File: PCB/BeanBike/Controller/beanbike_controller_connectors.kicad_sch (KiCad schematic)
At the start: 12 parts, among them J2 Motor Conn, J3 Throttle Conn, J4 PAS Conn, J5 Display Conn, J6 Brake Conn, J7 DEBUG Conn

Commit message: Footprints
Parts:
- J2: footprint (none) -> Connector_PinHeader_2.54mm:PinHeader_1x08_P2.54mm_Vertical
- J3, J4, J7: footprint (none) -> Connector_PinHeader_2.54mm:PinHeader_1x03_P2.54mm_Vertical
- J5: footprint (none) -> Connector_PinHeader_2.54mm:PinHeader_1x06_P2.54mm_Vertical
- J6: footprint (none) -> Connector_PinHeader_2.54mm:PinHeader_1x02_P2.54mm_Vertical
- R10, R6, R8: footprint (none) -> Resistor_SMD:R_0805_2012Metric; LCSC C98220 -> C17414
- R11, R7, R9: footprint (none) -> Resistor_SMD:R_0805_2012Metric; LCSC C137655 -> C17506
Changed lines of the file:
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@@
 			)
 		)
-		(property "Footprint" ""
+		(property "Footprint" "Resistor_SMD:R_0805_2012Metric"
 			(at 212.598 27.94 90)
 			(effects
@@
 			)
 		)
-		(property "LCSC" "C137655"
+		(property "LCSC" "C17506"
 			(at 210.82 27.94 0)
 			(effects
@@
 			)
 		)
-		(property "Footprint" ""
+		(property "Footprint" "Resistor_SMD:R_0805_2012Metric"
 			(at 211.328 48.26 90)
 			(effects
@@
 			)
 		)
-		(property "LCSC" "C137655"
+		(property "LCSC" "C17506"
 			(at 209.55 48.26 0)
 			(effects
@@
 			)
 		)
-		(property "Footprint" ""
+		(property "Footprint" "Resistor_SMD:R_0805_2012Metric"
 			(at 199.39 53.848 90)
 			(effects
@@
 			)
 		)
-		(property "LCSC" "C98220"
+		(property "LCSC" "C17414"
 			(at 199.39 52.07 90)
 			(effects
@@
 			)
 		)
-		(property "Footprint" ""
+		(property "Footprint" "Resistor_SMD:R_0805_2012Metric"
 			(at 200.66 33.528 90)
 			(effects
@@
 			)
 		)
-		(property "LCSC" "C98220"
+		(property "LCSC" "C17414"
 			(at 200.66 31.75 90)
 			(effects
@@
 			)
 		)
-		(property "Footprint" ""
+		(property "Footprint" "Connector_PinHeader_2.54mm:PinHeader_1x08_P2.54mm_Vertical"
 			(at 54.61 139.7 0)
 			(effects
@@
 			)
 		)
-		(property "Footprint" ""
+		(property "Footprint" "Connector_PinHeader_2.54mm:PinHeader_1x03_P2.54mm_Vertical"
 			(at 121.92 139.7 0)
 			(effects
@@
 			)
 		)
-		(property "Footprint" ""
+		(property "Footprint" "Connector_PinHeader_2.54mm:PinHeader_1x03_P2.54mm_Vertical"
 			(at 92.71 139.7 0)
 			(effects
@@
 			)
 		)
-		(property "Footprint" ""
+		(property "Footprint" "Connector_PinHeader_2.54mm:PinHeader_1x02_P2.54mm_Vertical"
 			(at 186.69 139.7 0)
 			(effects
@@
 			)
 		)
-		(property "Footprint" ""
+		(property "Footprint" "Resistor_SMD:R_0805_2012Metric"
 			(at 199.39 71.628 90)
 			(effects
@@
 			)
 		)
-		(property "LCSC" "C98220"
+		(property "LCSC" "C17414"
 			(at 199.39 69.85 90)
 			(effects
@@
 			)
 		)
-		(property "Footprint" ""
+		(property "Footprint" "Resistor_SMD:R_0805_2012Metric"
 			(at 211.328 66.04 90)
 			(effects
@@
 			)
 		)
-		(property "LCSC" "C137655"
+		(property "LCSC" "C17506"
 			(at 209.55 66.04 0)
 			(effects
@@
 			)
 		)
-		(property "Footprint" ""
+		(property "Footprint" "Connector_PinHeader_2.54mm:PinHeader_1x06_P2.54mm_Vertical"
 			(at 156.21 139.7 0)
 			(effects
@@
 			)
 		)
-		(property "Footprint" ""
+		(property "Footprint" "Connector_PinHeader_2.54mm:PinHeader_1x03_P2.54mm_Vertical"
 			(at 217.17 139.7 0)
 			(effects

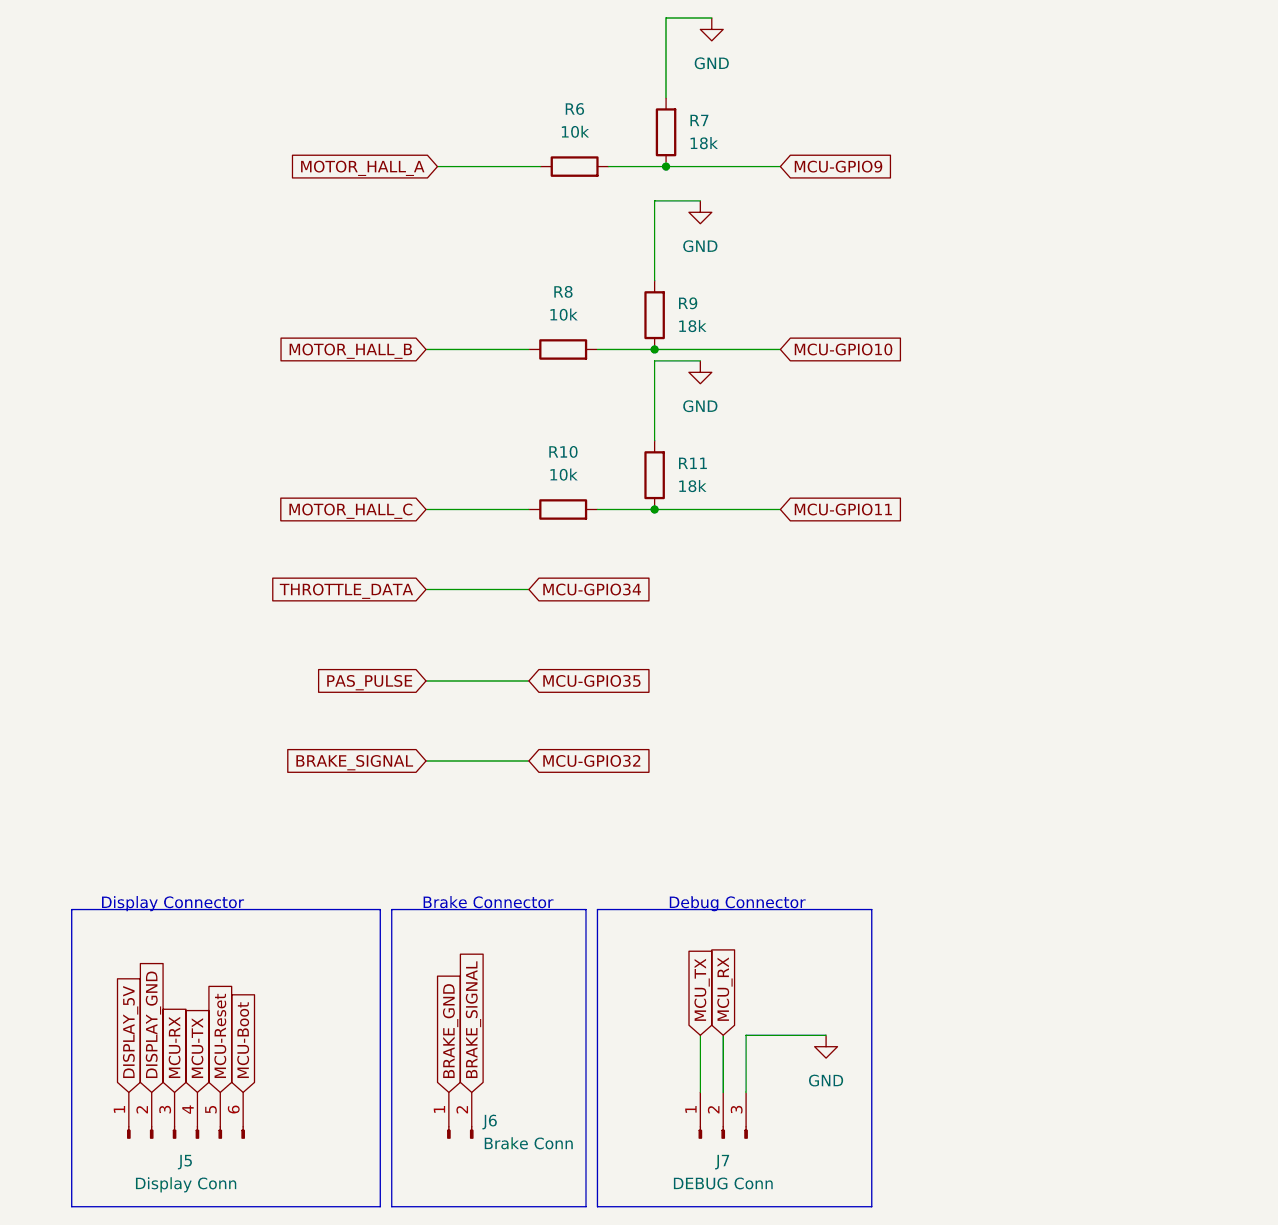
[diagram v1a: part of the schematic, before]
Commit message: PCB v3
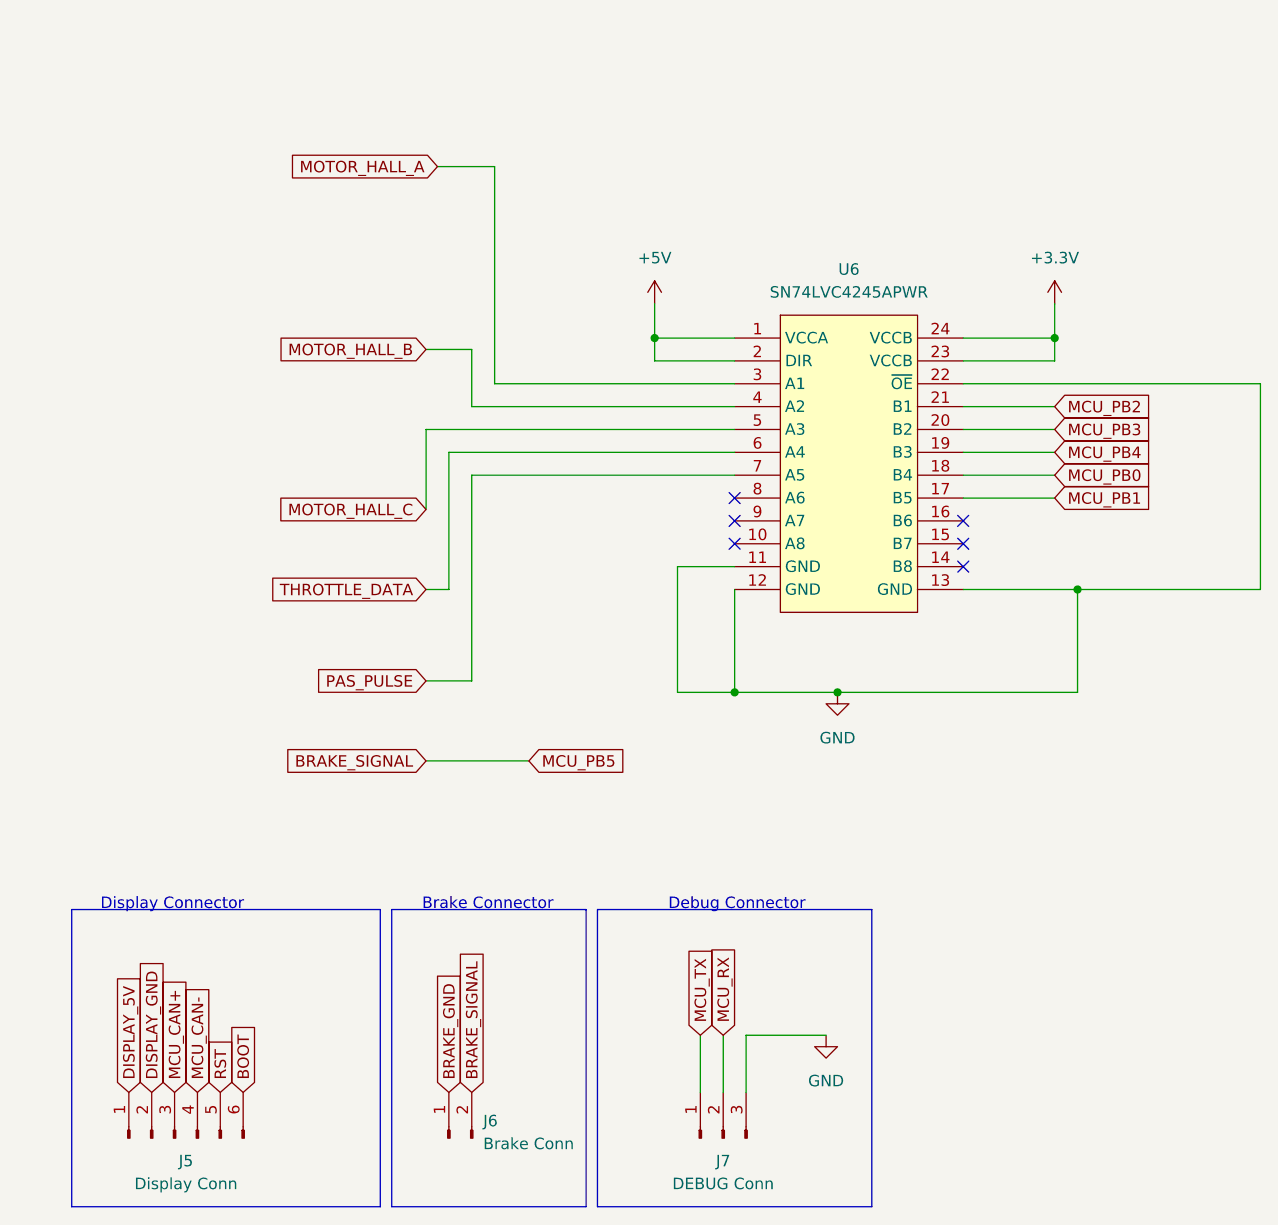
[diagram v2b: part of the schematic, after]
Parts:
- removed R10, R6, R8: 10k, Resistor_SMD:R_0805_2012Metric, symbol Device:R
- removed R11, R7, R9: 18k, Resistor_SMD:R_0805_2012Metric, symbol Device:R
- added U6: SN74LVC4245APWR, easyeda2kicad:TSSOP-24_L7.8-W4.4-P0.65-LS6.4-BL, symbol easyeda2kicad:SN74LVC4245APWR
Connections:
- net +5V: now also U6.1 (VCCA), U6.2 (DIR)
- net GND: now also U6.11 (GND), U6.12 (GND), U6.13 (GND), U6.22 (~{OE})
- net MOTOR_HALL_A: now also U6.3 (A1)
- net MOTOR_HALL_B: now also U6.4 (A2)
- net MOTOR_HALL_C: now also U6.5 (A3)
- net MCU-Boot renamed BOOT
- net MCU-GPIO34 renamed THROTTLE_DATA
- net THROTTLE_DATA: now also U6.6 (A4)
- net MCU-GPIO35 renamed PAS_PULSE
- net PAS_PULSE: now also U6.7 (A5)
- net MCU-RX renamed MCU_CAN+
- net MCU-Reset renamed RST
- net MCU-TX renamed MCU_CAN-
- new net +3.3V: U6.23 (VCCB), U6.24 (VCCB)
- new net MCU_PB0: U6.18 (B4)
- new net MCU_PB1: U6.17 (B5)
- new net MCU_PB2: U6.21 (B1)
- new net MCU_PB3: U6.20 (B2)
- new net MCU_PB4: U6.19 (B3)
- no-connect marks 0 -> 6

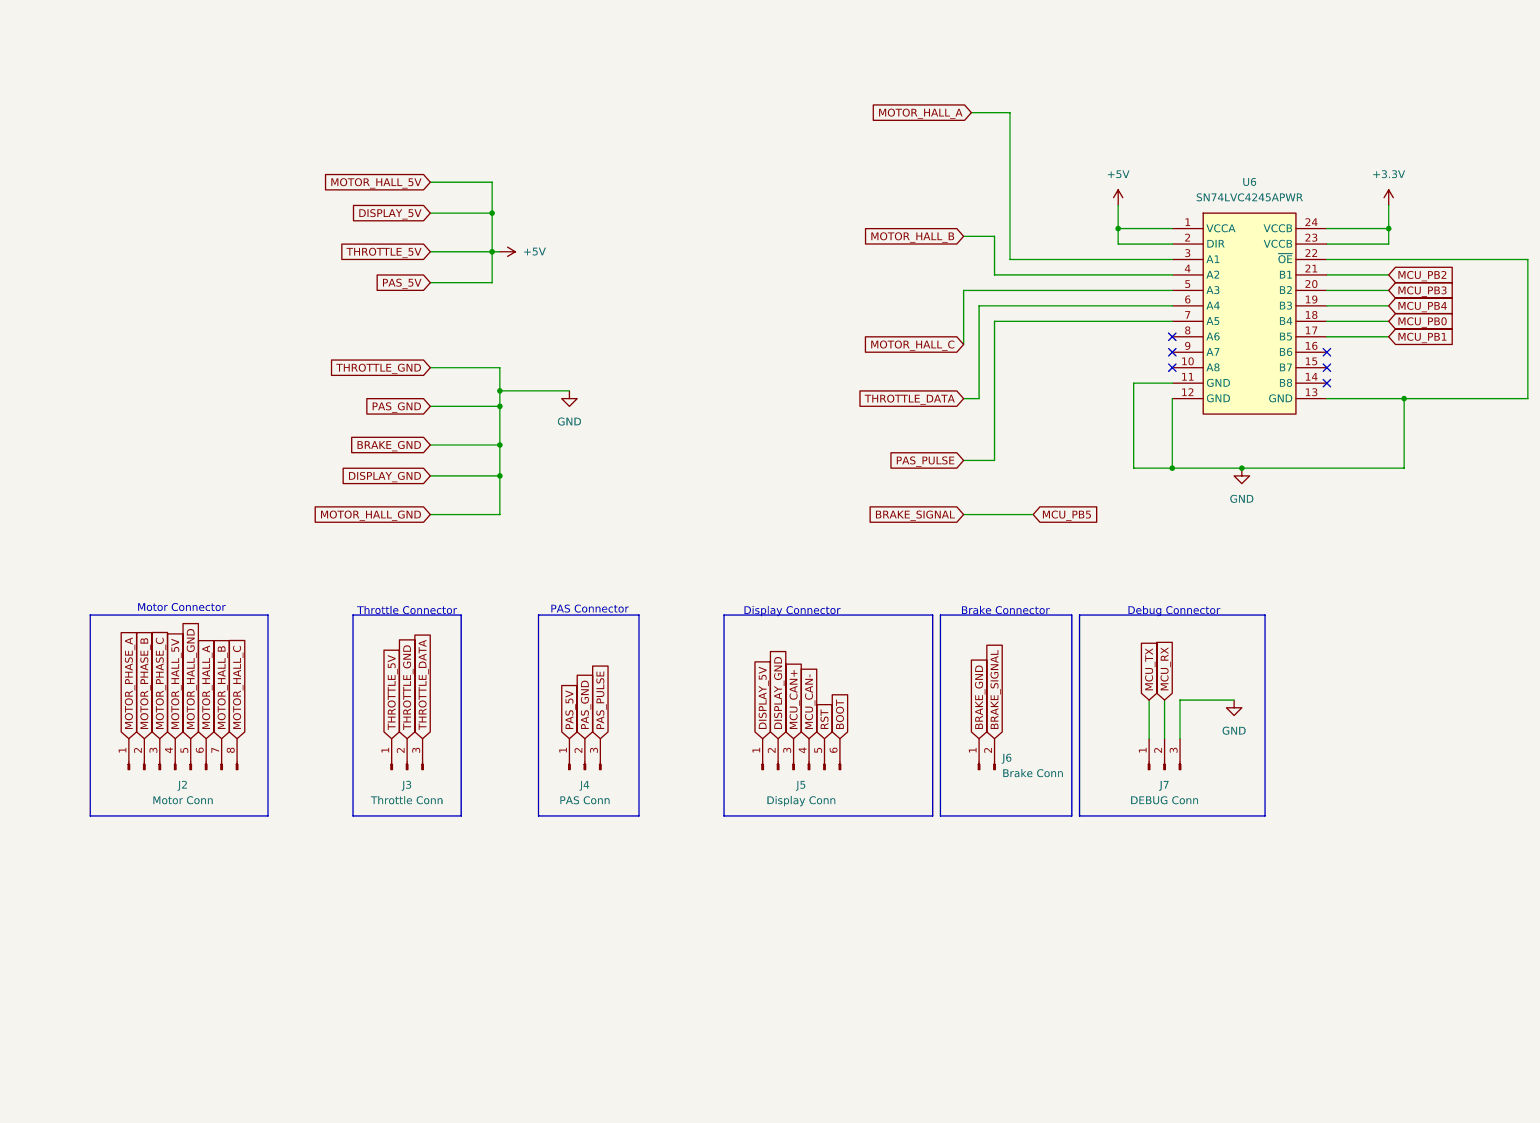
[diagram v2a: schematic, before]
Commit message: PCB v3
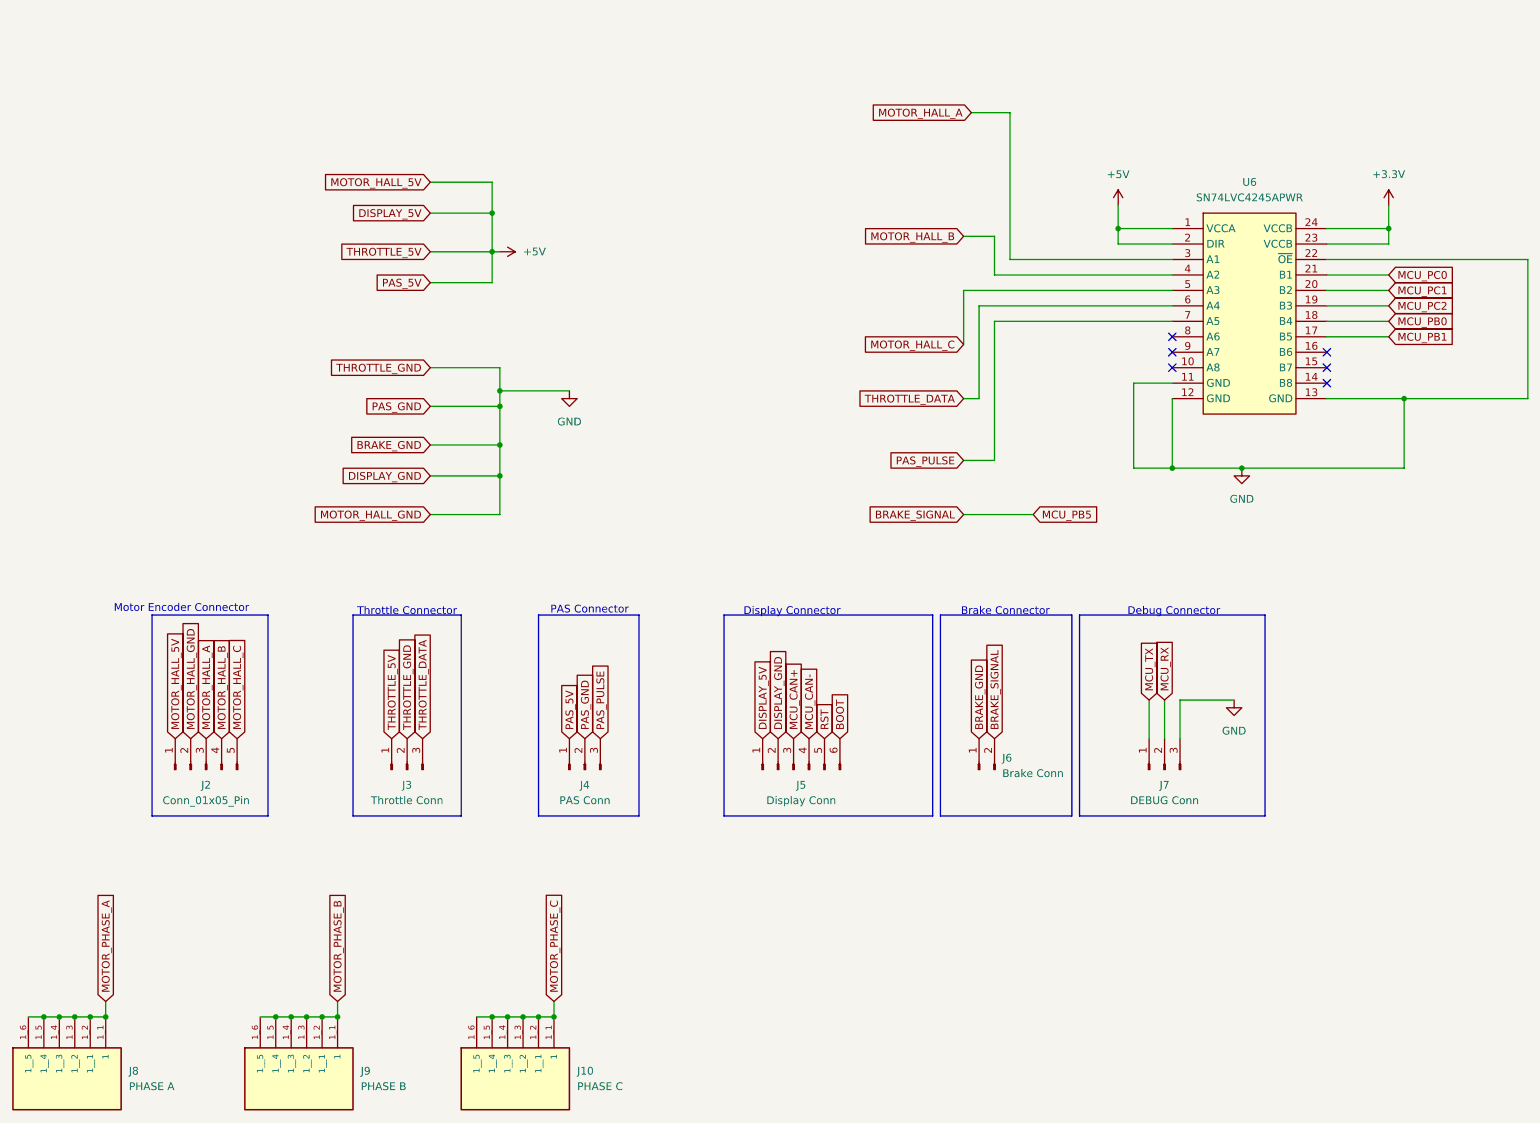
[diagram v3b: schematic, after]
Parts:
- removed J2: Motor Conn, Connector_PinHeader_2.54mm:PinHeader_1x08_P2.54mm_Vertical, symbol Connector:Conn_01x08_Pin
- added J10: PHASE C, 8196:KEYSTONE_8196, symbol 8196:8196
- added J2: Conn_01x05_Pin, Connector_PinHeader_2.54mm:PinHeader_1x05_P2.54mm_Vertical, symbol Connector:Conn_01x05_Pin
- added J8: PHASE A, 8196:KEYSTONE_8196, symbol 8196:8196
- added J9: PHASE B, 8196:KEYSTONE_8196, symbol 8196:8196
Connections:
- net +5V: now also J2.1 (Pin_1)
- net GND: now also J2.2 (Pin_2)
- net MOTOR_HALL_A: now also J2.3 (Pin_3)
- net MOTOR_HALL_B: now also J2.4 (Pin_4)
- net MOTOR_HALL_C: now also J2.5 (Pin_5)
- net MOTOR_PHASE_A: now also J8.1_1 (1), J8.1_2 (1__1), J8.1_3 (1__2), J8.1_4 (1__3), J8.1_5 (1__4), J8.1_6 (1__5)
- net MOTOR_PHASE_B: now also J9.1_1 (1), J9.1_2 (1__1), J9.1_3 (1__2), J9.1_4 (1__3), J9.1_5 (1__4), J9.1_6 (1__5)
- net MOTOR_PHASE_C: now also J10.1_1 (1), J10.1_2 (1__1), J10.1_3 (1__2), J10.1_4 (1__3), J10.1_5 (1__4), J10.1_6 (1__5)
- net MCU_PB2 renamed MCU_PC0
- net MCU_PB3 renamed MCU_PC1
- net MCU_PB4 renamed MCU_PC2
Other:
- note added: "Motor Encoder Connector"
- note removed: "Motor Connector"

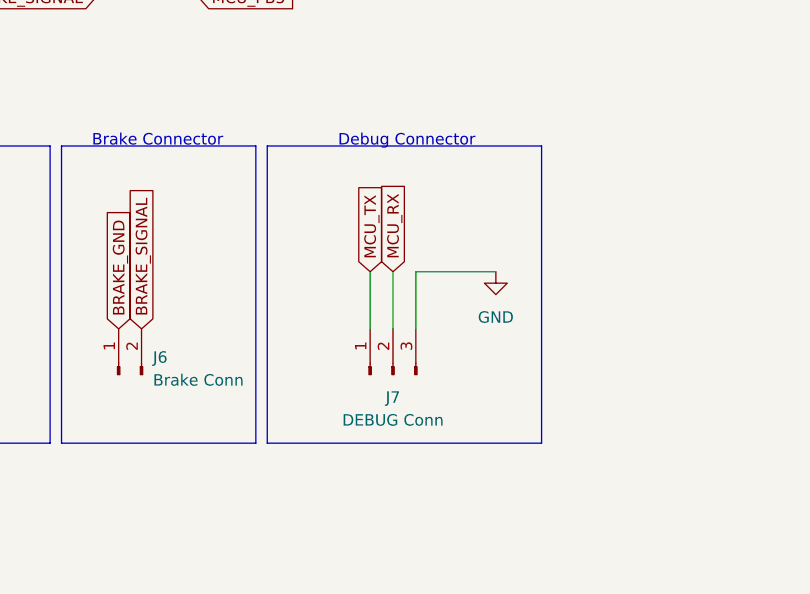
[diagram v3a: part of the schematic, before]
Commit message: big ol update
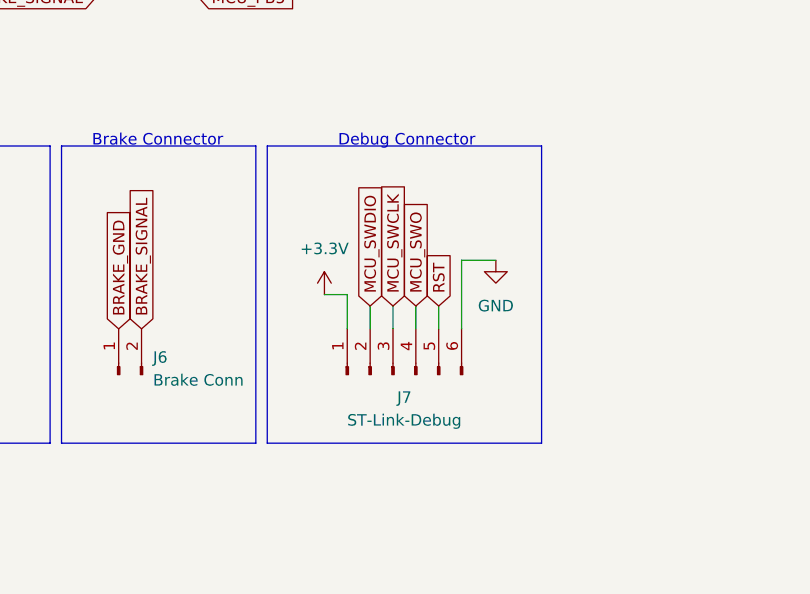
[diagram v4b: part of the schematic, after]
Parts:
- removed J7: DEBUG Conn, Connector_PinHeader_2.54mm:PinHeader_1x03_P2.54mm_Vertical, symbol Connector:Conn_01x03_Pin
- added J7: ST-Link-Debug, Connector_PinHeader_2.54mm:PinHeader_1x06_P2.54mm_Vertical, symbol Connector:Conn_01x06_Pin
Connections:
- net +3.3V: now also J7.1 (Pin_1)
- net GND: now also J7.6 (Pin_6)
- net RST: now also J7.5 (Pin_5)
- new net MCU_SWCLK: J7.3 (Pin_3)
- new net MCU_SWDIO: J7.2 (Pin_2)
- new net MCU_SWO: J7.4 (Pin_4)
